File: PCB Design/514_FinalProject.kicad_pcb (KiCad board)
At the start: 2 copper layers, 61 x 51 mm, 13 parts, among them J1 Conn_01x04_Pin, J2 Conn_01x04_Pin, J3 Conn_01x04_Pin, J4 Conn_01x06_Pin, J5 Conn_01x02_Pin

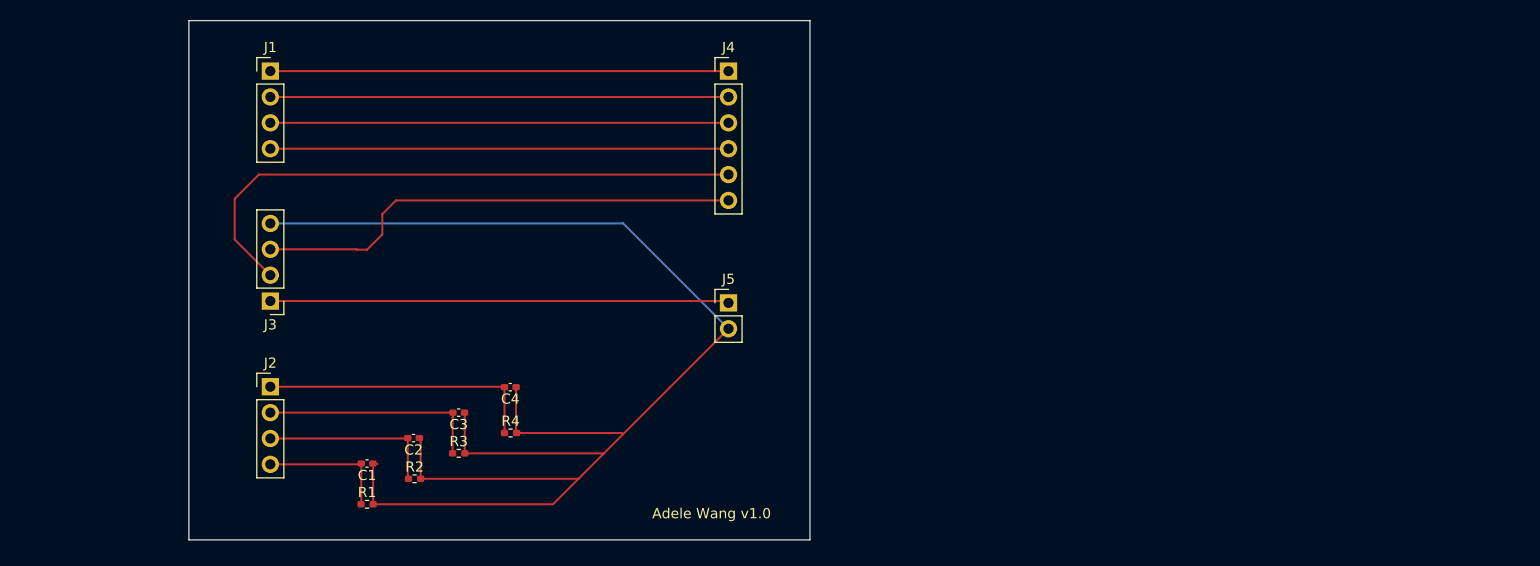
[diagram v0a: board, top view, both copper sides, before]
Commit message: codes
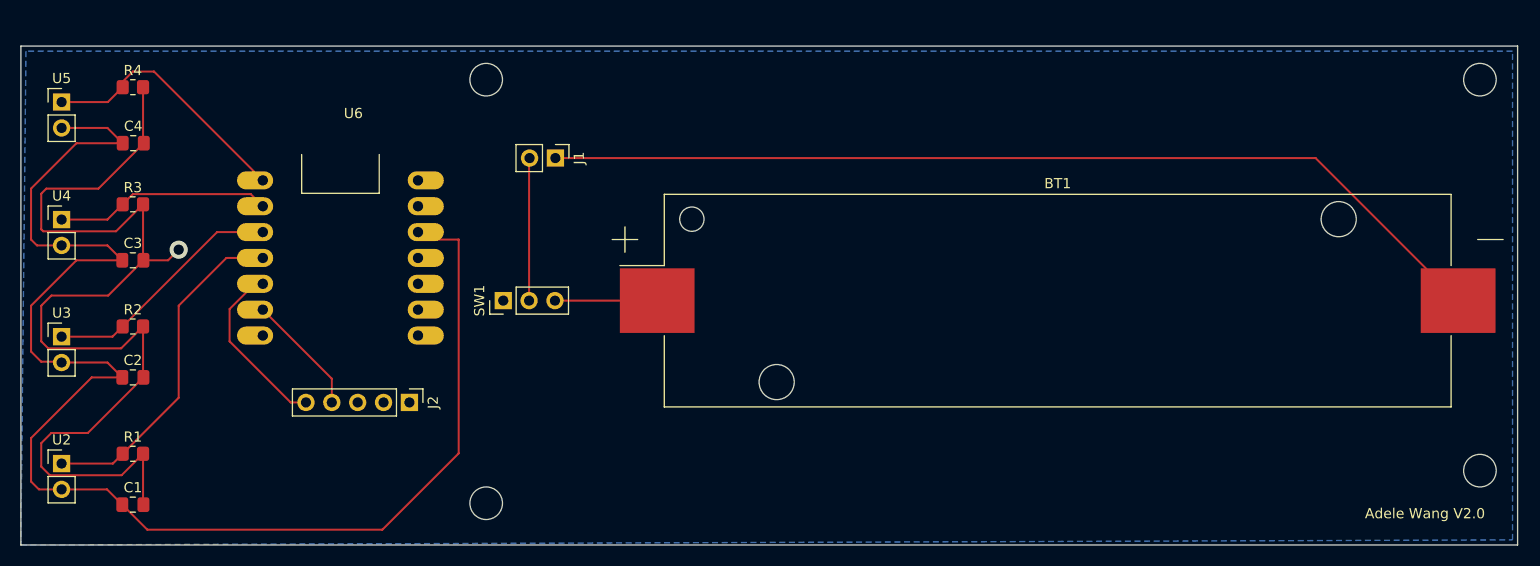
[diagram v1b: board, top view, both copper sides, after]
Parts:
- removed J3: Conn_01x04_Pin, Connector_PinHeader_2.54mm:PinHeader_1x04_P2.54mm_Vertical
- removed J4: Conn_01x06_Pin, Connector_PinHeader_2.54mm:PinHeader_1x06_P2.54mm_Vertical
- removed J5: Conn_01x02_Pin, Connector_PinHeader_2.54mm:PinHeader_1x02_P2.54mm_Vertical
- added BT1: Battery_Cell, Battery:BatteryHolder_Keystone_1042_1x18650, F.Cu at (179.3, 74.5)
- added SW1: SW_SPDT, Connector_PinHeader_2.54mm:PinHeader_1x03_P2.54mm_Vertical, F.Cu at (124.9, 74.5)
- added U2: FSR, Connector_PinHeader_2.54mm:PinHeader_1x02_P2.54mm_Vertical, F.Cu at (81.5, 90.5)
- added U3: FSR, Connector_PinHeader_2.54mm:PinHeader_1x02_P2.54mm_Vertical, F.Cu at (81.5, 78.0)
- added U4: FSR, Connector_PinHeader_2.54mm:PinHeader_1x02_P2.54mm_Vertical, F.Cu at (81.5, 66.5)
- added U5: FSR, Connector_PinHeader_2.54mm:PinHeader_1x02_P2.54mm_Vertical, F.Cu at (81.5, 55.0)
- added U6: ~, XIAO ESP32 S3:XIAO_ESP32_SENSE, F.Cu at (108.9, 70.3)
- C1, C2, C3, C4: value C -> 1uF; footprint Capacitor_SMD:C_0402_1005Metric_Pad0.74x0.62mm_HandSolder -> Capacitor_SMD:C_0805_2012Metric_Pad1.18x1.45mm_HandSolder
- J1: value Conn_01x04_Pin -> Conn_01x02_Socket; footprint Connector_PinHeader_2.54mm:PinHeader_1x04_P2.54mm_Vertical -> Connector_PinHeader_2.54mm:PinHeader_1x02_P2.54mm_Vertical
- J2: value Conn_01x04_Pin -> Conn_01x06_Socket; footprint Connector_PinHeader_2.54mm:PinHeader_1x04_P2.54mm_Vertical -> Connector_PinHeader_2.54mm:PinHeader_1x05_P2.54mm_Vertical
- R1, R2, R3, R4: value R -> 10k; footprint Resistor_SMD:R_0402_1005Metric_Pad0.72x0.64mm_HandSolder -> Resistor_SMD:R_0805_2012Metric_Pad1.20x1.40mm_HandSolder
- moved R4 50.3 mm to (88.5, 53.5)
- moved C4 44.1 mm to (88.5, 59.0), turned to 0 degrees
- moved R3 40.3 mm to (88.5, 65.0)
- moved C3 35.3 mm to (88.5, 70.5), turned to 0 degrees
- moved R2 31.5 mm to (88.5, 77.0)
- moved J1 29.3 mm to (130.0, 60.5), turned to -90 degrees
- moved C2 28.2 mm to (88.5, 82.0), turned to 0 degrees
- moved R1 23.5 mm to (88.5, 89.5)
- moved C1 23.4 mm to (88.5, 94.5), turned to 0 degrees
- moved J2 13.7 mm to (115.7, 84.5), turned to -90 degrees
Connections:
- C1 pad 1: GND -> +3V3
- C1 pad 2: Net-(J2-Pin_4) -> GND
- C2 pad 1: GND -> +3V3
- C2 pad 2: Net-(J2-Pin_3) -> GND
- C3 pad 1: GND -> +3V3
- C3 pad 2: Net-(J2-Pin_2) -> GND
- C4 pad 1: GND -> +3V3
- C4 pad 2: Net-(J2-Pin_1) -> GND
- J2 pad 1: Net-(J2-Pin_1) -> unconnected-(J2-Pin_1-Pad1)
- J2 pad 2: Net-(J2-Pin_2) -> +3.3V
- J2 pad 3: Net-(J2-Pin_3) -> GND
- R1 pad 1: Net-(J2-Pin_4) -> Net-(U2-VIN)
- R2 pad 1: Net-(J2-Pin_3) -> Net-(U3-VIN)
- R3 pad 1: Net-(J2-Pin_2) -> Net-(U4-VIN)
- R4 pad 1: Net-(J2-Pin_1) -> Net-(U5-VIN)
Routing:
- net +3V3: track 45.1 -> 145.7 mm
- net Net-(J3-Pin_2): track 58.4 -> 0.00 mm
- net Net-(BT1--): track 45.0 -> 94.5 mm
- net Net-(J3-Pin_3): track 48.2 -> 0.00 mm
- net Net-(J1-Pin_4): track 45.0 -> 0.00 mm
- net Net-(J1-Pin_3): track 45.0 -> 0.00 mm
- net GND: track 148.1 -> 104.6 mm, vias 0 -> 1
- net Net-(U2-VIN): track 0.00 -> 33.4 mm
- net Net-(J1-Pin_2): track 45.0 -> 14.0 mm
- net Net-(J2-Pin_1): track 27.5 -> 0.00 mm
- net Net-(U5-VIN): track 0.00 -> 25.8 mm
- net Net-(U3-VIN): track 0.00 -> 24.0 mm
- net Net-(J2-Pin_2): track 21.9 -> 0.00 mm
- net Net-(U4-VIN): track 0.00 -> 21.3 mm
- net Net-(J2-Pin_3): track 17.5 -> 0.00 mm
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- added copper zone on B.Cu, net GND
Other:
- board size 61 x 51 mm -> 147 x 49 mm
- board text added: "Adele Wang V2.0"
- board text removed: "Adele Wang v1.0"
